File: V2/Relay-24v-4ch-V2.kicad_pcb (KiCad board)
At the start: 2 copper layers, 68 x 67.8 mm, 21 parts, among them J1 DB141V-2.54-5P, J2 DB142V-5.08-2P, J3 DB142V-5.08-2P, J4 DB142V-5.08-2P, J5 DB142V-5.08-2P, K1 SRD-24VDC-SL-A, K2 SRD-24VDC-SL-A, K3 SRD-24VDC-SL-A, K4 SRD-24VDC-SL-A

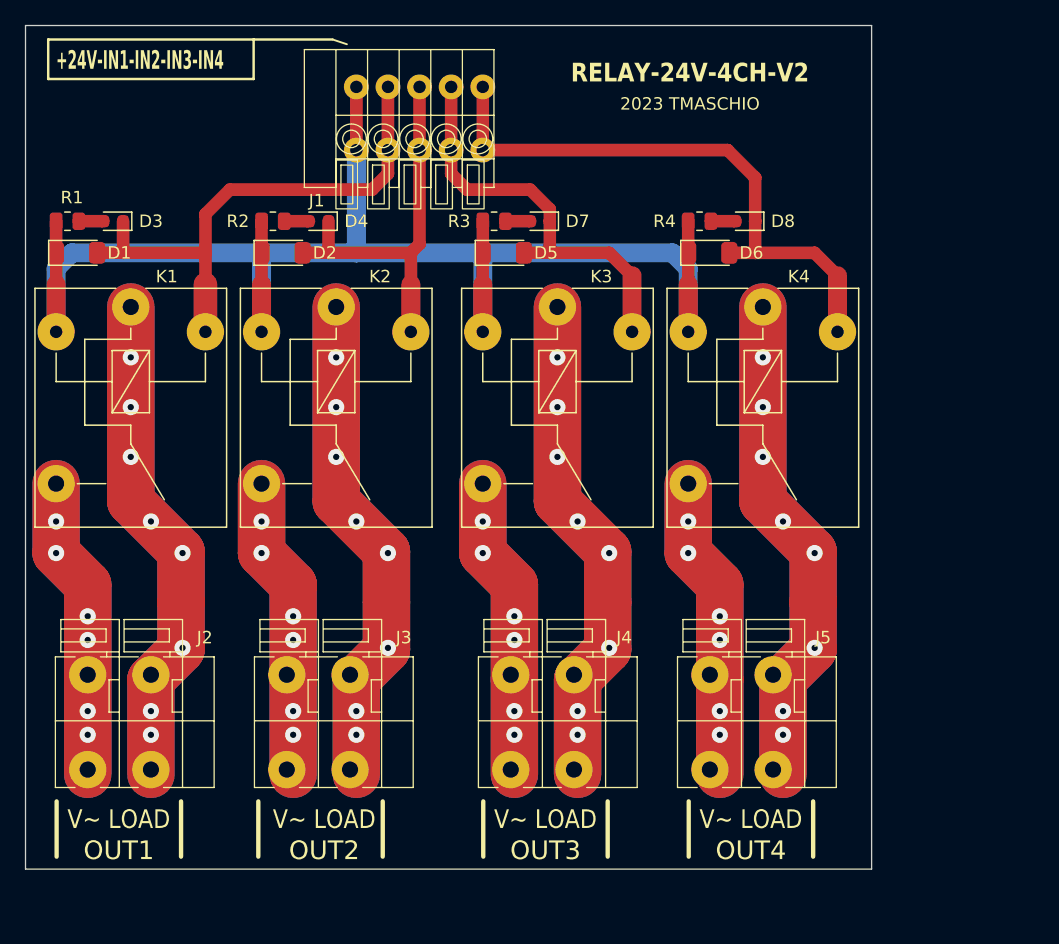
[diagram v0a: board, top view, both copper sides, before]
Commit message: Redone everything
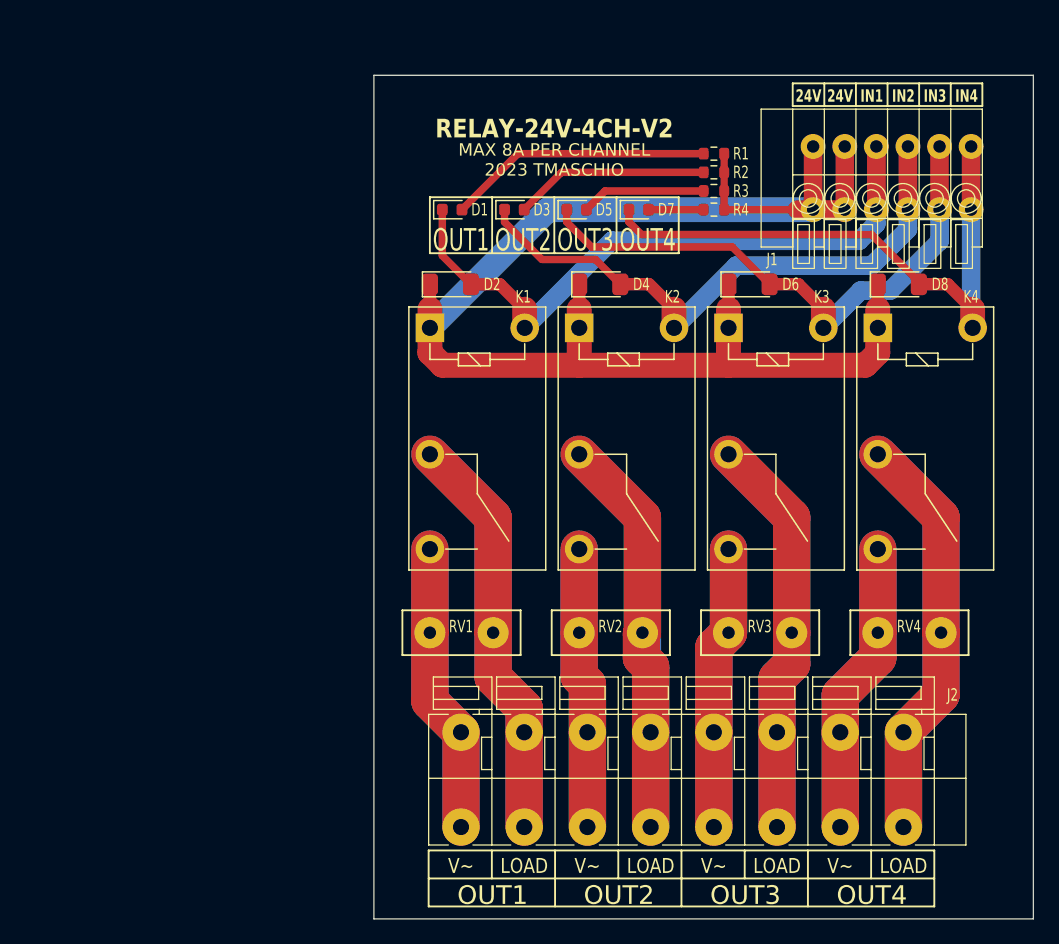
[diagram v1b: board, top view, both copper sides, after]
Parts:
- removed J3, J4, J5: DB142V-5.08-2P, Tales:TerminalBlock_Dibo_DB142V-5.08-2P_1x02_P5.08mm_Vertical
- added RV1: 275VAC, Tales:RV_Disc_D9.50mm_W3.6mm_P5.08mm, F.Cu at (129.5, 107.0)
- added RV2: 275VAC, Tales:RV_Disc_D9.50mm_W3.6mm_P5.08mm, F.Cu at (141.5, 107.0)
- added RV3: 275VAC, Tales:RV_Disc_D9.50mm_W3.6mm_P5.08mm, F.Cu at (153.5, 107.0)
- added RV4: 275VAC, Tales:RV_Disc_D9.50mm_W3.6mm_P5.08mm, F.Cu at (165.5, 107.0)
- D1: renamed from D3; value GREEN/0603 -> GREEN
- D2: renamed from D1; value 1N4148/SOD-123 -> 1N4148
- D3: renamed from D4; value GREEN/0603 -> GREEN
- D4: renamed from D2; value 1N4148/SOD-123 -> 1N4148
- D5: renamed from D7; value GREEN/0603 -> GREEN
- D6: renamed from D5; value 1N4148/SOD-123 -> 1N4148
- D7: renamed from D8; value GREEN/0603 -> GREEN
- D8: renamed from D6; value 1N4148/SOD-123 -> 1N4148
- J1: value DB141V-2.54-5P -> DG141V-2.54-6P; footprint Tales:TerminalBlock_Dibo_DB141V-2.54-5P_1x05_P2.54mm_Vertical -> Tales:TerminalBlock_Dibo_DB141V-2.54-6P_1x06_P2.54mm_Vertical
- J2: value DB142V-5.08-2P -> DB142V-5.08-8P; footprint Tales:TerminalBlock_Dibo_DB142V-5.08-2P_1x02_P5.08mm_Vertical -> Tales:TerminalBlock_Dibo_DB142V-5.08-8P_1x08_P5.08mm_Vertical
- K1, K2, K3, K4: value SRD-24VDC-SL-A -> G5Q-1A4-DC24V; footprint Tales:Relay_SPST_Songle_SRD_FormA -> Tales:Relay_SPST_Omron-G5Q-1A
- R1, R2, R3, R4: value 4k7/0,125W/0805 -> 5k6/100mW; footprint Tales:R_0805_2012Metric -> Tales:R_0603_1608Metric
- moved R1 52.2 mm to (152.3, 68.5), turned to 180 degrees
- moved J1 39.5 mm to (173.0, 67.9)
- moved R2 35.7 mm to (152.3, 70.0), turned to 180 degrees
- moved J2 30.4 mm to (132.0, 122.6)
- moved D2 30.1 mm to (131.2, 79.0)
- moved D1 27.2 mm to (131.3, 73.0), turned to 0 degrees
- moved D4 25.7 mm to (143.2, 79.0)
- moved K1 24.1 mm to (129.5, 82.5)
- moved D6 19.9 mm to (155.2, 79.0)
- moved K2 19.6 mm to (141.5, 82.5)
- moved R3 17.8 mm to (152.3, 71.5), turned to 180 degrees
- moved D3 15.7 mm to (136.3, 73.0), turned to 0 degrees
- moved D8 15.4 mm to (167.2, 79.0)
- moved K3 13.9 mm to (153.5, 82.5)
- moved K4 9.39 mm to (165.5, 82.5)
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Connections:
- D1 pad 1: Net-(D1-A) (its old number) -> Net-(D1-K)
- D2 pad 2: Net-(D1-A) (its old number) -> Net-(D1-K)
- D3 pad 1: Net-(D2-A) -> Net-(D3-K)
- D4 pad 2: Net-(D2-A) -> Net-(D3-K)
- D5 pad 1: Net-(D5-A) (its old number) -> Net-(D5-K)
- D6 pad 2: Net-(D5-A) (its old number) -> Net-(D5-K)
- D7 pad 1: Net-(D6-A) -> Net-(D7-K)
- D8 pad 2: Net-(D6-A) -> Net-(D7-K)
- J1 pad 1: Net-(D6-A) -> Net-(D7-K)
- J1 pad 2: Net-(D5-A) (its old number) -> Net-(D5-K)
- J1 pad 3: Net-(D2-A) -> Net-(D3-K)
- J1 pad 4: Net-(D1-A) (its old number) -> Net-(D1-K)
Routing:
- net Net-(J5-Pin_2): track 80.5 -> 0.00 mm, vias 8 -> 0
- net Net-(J3-Pin_2): track 80.5 -> 0.00 mm, vias 8 -> 0
- net Net-(J4-Pin_2): track 80.5 -> 0.00 mm, vias 8 -> 0
- net Net-(J2-Pin_8): track 0.00 -> 66.6 mm
- net Net-(J2-Pin_6): track 0.00 -> 65.1 mm
- net Net-(J2-Pin_4): track 0.00 -> 64.8 mm
- net Net-(D1-K): track 0.00 -> 51.5 mm
- net Net-(J5-Pin_1): track 48.8 -> 0.00 mm, vias 6 -> 0
- net Net-(J3-Pin_1): track 48.8 -> 0.00 mm, vias 6 -> 0
- net Net-(J4-Pin_1): track 48.8 -> 0.00 mm, vias 6 -> 0
- net Net-(D6-A): track 47.9 -> 0.00 mm
- net Net-(D7-K): track 0.00 -> 47.8 mm
- net Net-(D3-K): track 0.00 -> 47.8 mm
- net Net-(J2-Pin_7): track 0.00 -> 47.2 mm
- net Net-(D5-K): track 0.00 -> 45.9 mm
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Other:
- board size 68 x 67.8 mm -> 53 x 67.8 mm
- board text added: "24V"
- board text added: "CORRENTE MÁXIMA POR CANAL CONSIDERAÇÕES: - ESPESSURA COBRE 0,035mm, TRILHAS EM AMBOS LAYERS, EQUIVALE 0,070mm - deltaT NA TRILHA 10ºC - LARGURA DE TRILHA NECESSÁRIA PARA 8A = 2,64418mm TRILHAS DESENHADAS EM AMBOS OS LAYERS COM 3,0mm DE LARGURA LIMITE DE 8A ESTABELECIDO PARA PRESERVAÇÃO DO RELÊ"
- board text added: "IN1"
- board text added: "IN2"
- board text added: "IN3"
- board text added: "IN4"
- board text added: "LOAD"
- board text added: "MAX 8A PER CHANNEL 2023 TMASCHIO"
- board text added: "V~"
- board text removed: "+24V-IN1-IN2-IN3-IN4"
- board text removed: "2023 TMASCHIO"
- board text removed: "V~ LOAD"
